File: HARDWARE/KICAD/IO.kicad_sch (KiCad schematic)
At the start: 18 parts, among them J1 Conn_01x20_Socket, J4 USB_C_Receptacle_USB2.0_16P, J5 Micro_SD_Card, J6 Conn_01x20_Socket, U5 USBLC6-2SC6

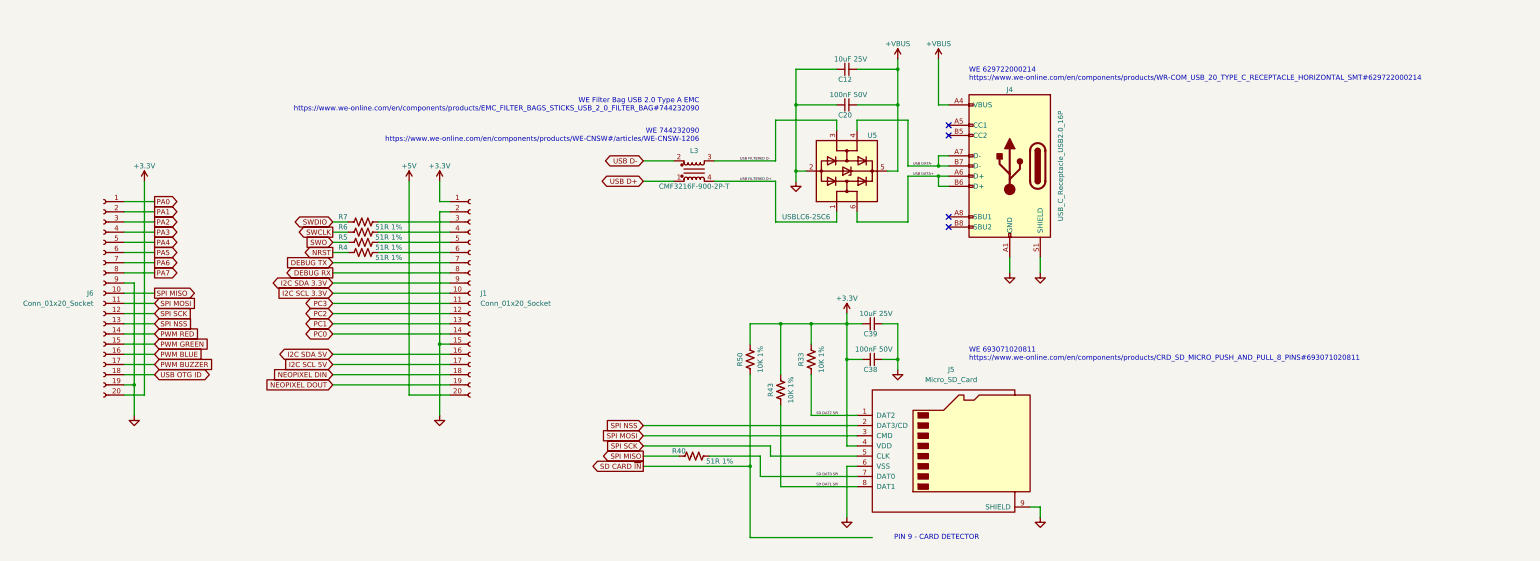
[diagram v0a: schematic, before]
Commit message: Improvements to layout. Fixed most of errors and warnings. Added correct footprint for Micro SD socket. Added markings and symbols to legend.
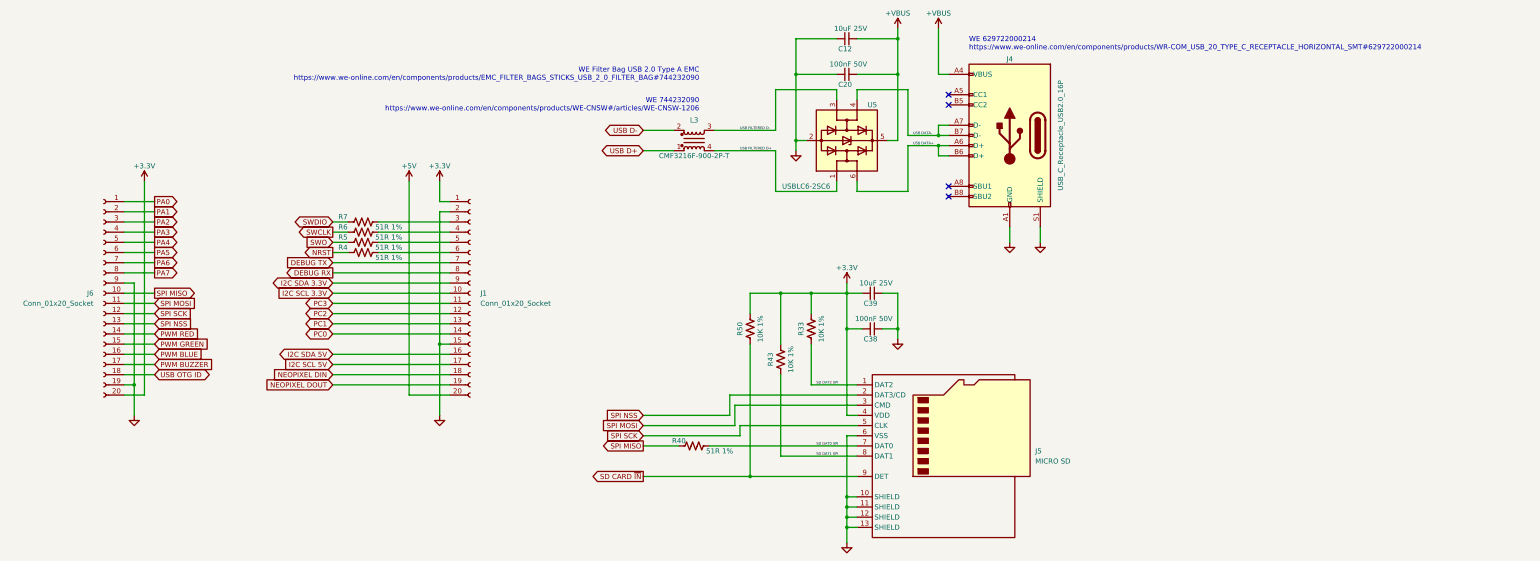
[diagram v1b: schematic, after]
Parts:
- removed J5: Micro_SD_Card, Connector_Card:microSD_HC_Wuerth_693072010801, symbol Connector:Micro_SD_Card
- added J5: MICRO SD, STM32XP:WE 693071020811, symbol STM32XP:WE_693071020811
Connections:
- net +3.3V: now also J5.4 (VDD)
- net GND: now also J5.10 (SHIELD), J5.11 (SHIELD), J5.12 (SHIELD), J5.13 (SHIELD), J5.6 (VSS)
- net SD CARD ~{IN}: now also J5.9 (DET)
- net SD DAT0 SPI: now also J5.7 (DAT0)
- net SD DAT1 SPI: now also J5.8 (DAT1)
- net SD DAT2 SPI: now also J5.1 (DAT2)
- net SPI MOSI: now also J5.3 (CMD)
- net SPI NSS: now also J5.2 (DAT3/CD)
- net SPI SCK: now also J5.5 (CLK)
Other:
- note removed: "PIN 9 - CARD DETECTOR"
- note removed: "WE 693071020811 https://www.we-online.com/en/components/products/CRD_SD_MICRO_PUSH_AND_PULL_8_PINS#693071020811"
- moved on the sheet: C12, C20, C38, C39, J4, L3, R33, R40, R43, R50, U5
